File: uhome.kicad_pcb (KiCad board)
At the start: 2 copper layers, 26 x 25.5 mm, 290 parts, among them J1 C2, J2 ANT, U1 Si7006, U2 LPS22HB, U3 EFM8SB10, U4 Si4012, U5 AH1806

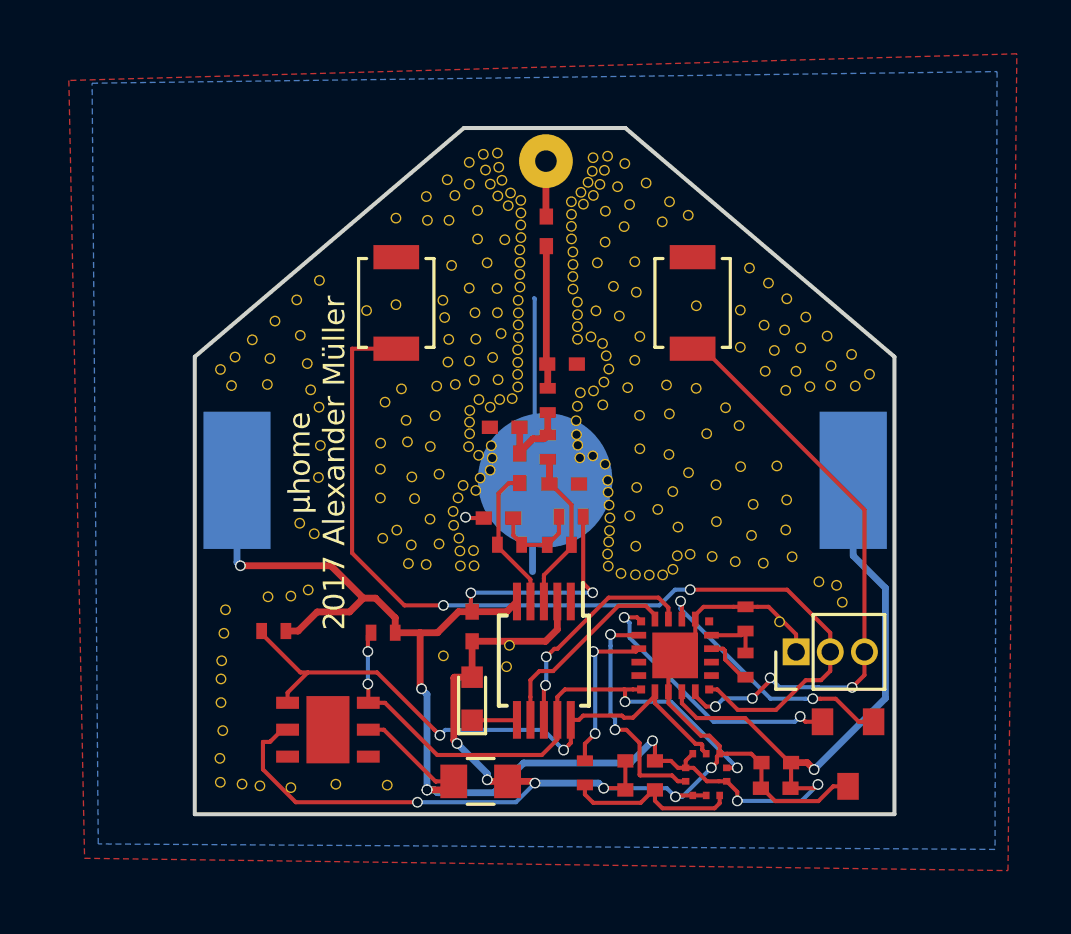
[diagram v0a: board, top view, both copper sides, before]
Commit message: Revision 2
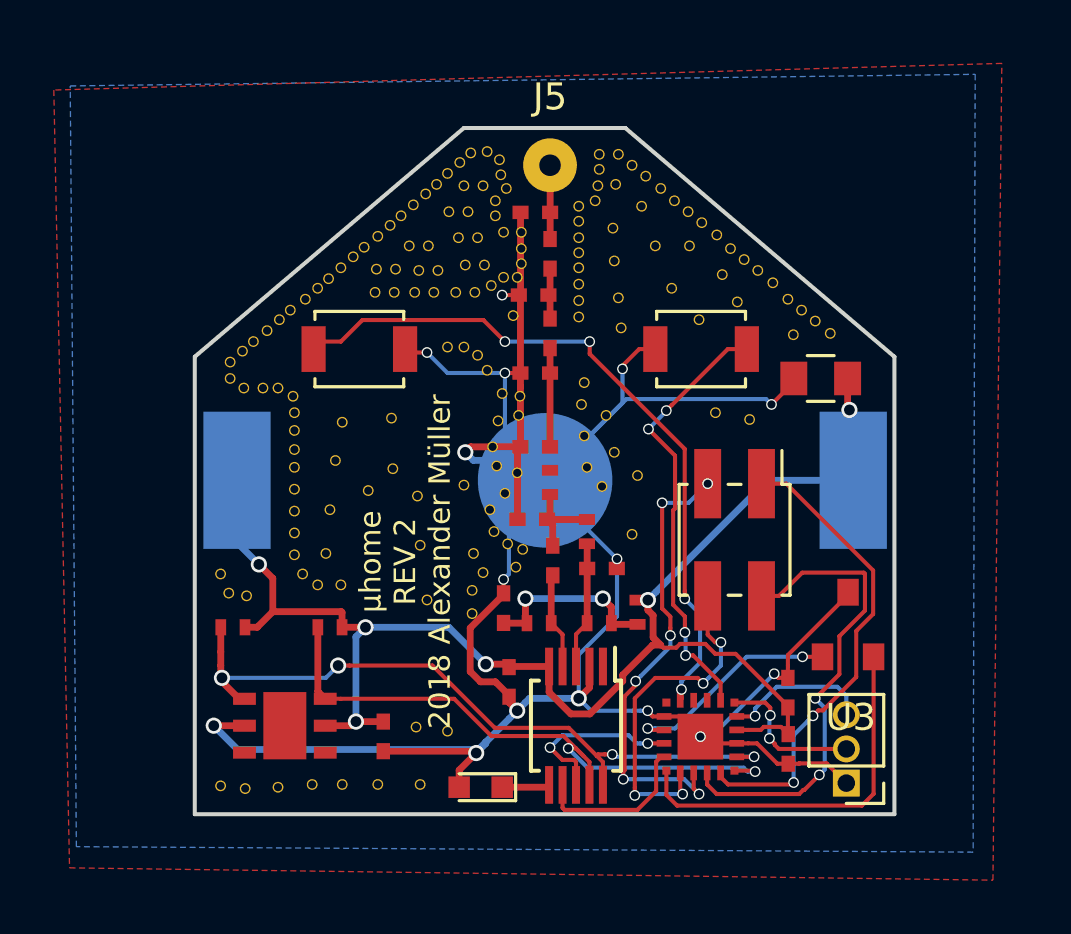
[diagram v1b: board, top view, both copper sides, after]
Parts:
- removed the ? at (173.7, 142.8)
- removed the ? at (152.9, 148.8)
- removed the ? at (159.5, 127.8)
- removed the ? at (169.6, 136.6)
- removed the ? at (169.6, 135.1)
- removed the ? at (168.5, 135.2)
- removed the ? at (168.5, 136.4)
- removed the ? at (168.4, 137.9)
- removed the ? at (168.2, 138.9)
- removed the ? at (169.2, 138.7)
- removed the ? at (169.8, 138.0)
- removed the ? at (170.3, 137.3)
- removed the ? at (152.9, 147.9)
- removed the ? at (171.0, 135.9)
- removed the ? at (171.4, 137.8)
- removed the ? at (172.3, 137.1)
- removed the ? at (171.4, 139.1)
- removed the ? at (172.8, 138.5)
- removed the ? at (172.7, 139.6)
- removed the ? at (170.0, 139.3)
- removed the ? at (168.4, 140.0)
- removed the ? at (169.9, 140.4)
- removed the ? at (170.4, 140.3)
- removed the ? at (153.0, 146.9)
- removed the ? at (171.2, 140.4)
- removed the ? at (172.1, 140.6)
- removed the ? at (173.1, 140.7)
- removed the ? at (175.2, 141.4)
- removed the ? at (176.1, 142.1)
- removed the ? at (175.8, 141.5)
- removed the ? at (174.2, 140.4)
- removed the ? at (174.0, 139.4)
- removed the ? at (174.0, 138.3)
- removed the ? at (173.6, 137.1)
- removed the ? at (153.0, 145.9)
- removed the ? at (172.2, 135.6)
- removed the ? at (171.7, 134.9)
- removed the ? at (170.6, 134.2)
- removed the ? at (169.5, 134.1)
- removed the ? at (168.1, 134.1)
- removed the ? at (167.2, 134.8)
- removed the ? at (161.1, 140.0)
- removed the ? at (160.7, 139.0)
- removed the ? at (160.2, 138.3)
- removed the ? at (160.1, 137.5)
- removed the ? at (153.0, 145.0)
- removed the ? at (161.1, 137.4)
- removed the ? at (160.8, 136.3)
- removed the ? at (159.9, 136.2)
- removed the ? at (159.9, 135.4)
- removed the ? at (160.9, 135.2)
- removed the ? at (161.0, 134.1)
- removed the ? at (159.7, 134.2)
- removed the ? at (159.1, 134.7)
- removed the ? at (158.9, 136.2)
- removed the ? at (158.9, 137.2)
- removed the ? at (153.0, 144.3)
- removed the ? at (158.9, 138.2)
- removed the ? at (159.9, 140.7)
- removed the ? at (159.0, 139.7)
- removed the ? at (159.5, 139.4)
- removed the ? at (160.0, 140.0)
- removed the ? at (160.6, 140.7)
- removed the ? at (156.3, 134.2)
- removed the ? at (156.6, 134.9)
- removed the ? at (156.7, 136.3)
- removed the ? at (156.6, 137.5)
- removed the ? at (153.1, 143.3)
- removed the ? at (155.9, 139.2)
- removed the ? at (156.4, 139.6)
- removed the ? at (162.6, 134.6)
- removed the ? at (162.2, 135.0)
- removed the ? at (162.2, 135.4)
- removed the ? at (162.2, 135.9)
- removed the ? at (162.2, 136.3)
- removed the ? at (162.5, 136.7)
- removed the ? at (167.3, 125.5)
- removed the ? at (167.2, 126.1)
- removed the ? at (153.1, 142.4)
- removed the ? at (167.1, 126.6)
- removed the ? at (166.8, 127.0)
- removed the ? at (162.7, 125.5)
- removed the ? at (162.8, 126.1)
- removed the ? at (163.0, 126.6)
- removed the ? at (163.3, 127.0)
- removed the ? at (163.6, 127.4)
- removed the ? at (166.4, 127.3)
- removed the ? at (163.2, 125.4)
- removed the ? at (163.3, 126.0)
- removed the ? at (156.2, 141.7)
- removed the ? at (163.4, 126.4)
- removed the ? at (163.7, 126.9)
- removed the ? at (166.8, 125.6)
- removed the ? at (166.8, 126.1)
- removed the ? at (166.6, 126.5)
- removed the ? at (166.3, 126.9)
- removed the ? at (169.8, 140.9)
- removed the ? at (169.4, 141.1)
- removed the ? at (168.9, 141.1)
- removed the ? at (168.4, 141.1)
- removed the ? at (155.6, 141.9)
- removed the ? at (167.8, 141.1)
- removed the ? at (167.4, 140.8)
- removed the ? at (167.3, 140.3)
- removed the ? at (167.4, 139.9)
- removed the ? at (167.4, 139.5)
- removed the ? at (167.4, 139.0)
- removed the ? at (167.4, 138.5)
- removed the ? at (167.4, 138.0)
- removed the ? at (167.3, 137.6)
- removed the ? at (167.2, 137.0)
- removed the ? at (161.2, 144.1)
- removed the ? at (154.7, 141.9)
- removed the ? at (166.8, 136.7)
- removed the ? at (166.3, 136.8)
- removed the ? at (166.2, 136.3)
- removed the ? at (166.2, 135.9)
- removed the ? at (166.2, 135.4)
- removed the ? at (166.2, 134.8)
- removed the ? at (166.3, 134.3)
- removed the ? at (166.8, 134.3)
- removed the ? at (167.2, 133.9)
- removed the ? at (167.4, 133.5)
- removed the ? at (170.6, 131.1)
- removed the ? at (167.3, 133.0)
- removed the ? at (167.2, 132.5)
- removed the ? at (166.7, 132.3)
- removed the ? at (166.2, 132.3)
- removed the ? at (166.2, 131.9)
- removed the ? at (166.2, 131.4)
- removed the ? at (166.2, 131.0)
- removed the ? at (166.1, 130.5)
- removed the ? at (166.0, 130.0)
- removed the ? at (166.1, 129.6)
- removed the ? at (159.5, 131.1)
- removed the ? at (166.0, 129.1)
- removed the ? at (166.0, 128.6)
- removed the ? at (166.0, 128.2)
- removed the ? at (166.0, 127.7)
- removed the ? at (166.0, 127.2)
- removed the ? at (164.1, 128.6)
- removed the ? at (164.1, 128.1)
- removed the ? at (164.1, 127.7)
- removed the ? at (164.1, 127.2)
- removed the ? at (164.1, 130.4)
- removed the ? at (158.4, 131.3)
- removed the ? at (164.1, 129.9)
- removed the ? at (164.1, 129.5)
- removed the ? at (164.1, 129.0)
- removed the ? at (164.0, 132.3)
- removed the ? at (164.0, 131.8)
- removed the ? at (164.0, 131.4)
- removed the ? at (164.0, 130.9)
- removed the ? at (164.0, 133.2)
- removed the ? at (164.0, 132.7)
- removed the ? at (164.0, 133.7)
- removed the ? at (155.9, 132.2)
- removed the ? at (164.0, 134.1)
- removed the ? at (163.8, 134.6)
- removed the ? at (163.3, 134.6)
- removed the ? at (163.0, 134.9)
- removed the ? at (162.0, 137.8)
- removed the ? at (162.4, 138.0)
- removed the ? at (163.0, 136.3)
- removed the ? at (163.1, 136.8)
- removed the ? at (163.0, 137.2)
- removed the ? at (162.6, 137.5)
- removed the ? at (156.2, 133.3)
- removed the ? at (161.8, 138.2)
- removed the ? at (161.6, 138.7)
- removed the ? at (161.6, 139.3)
- removed the ? at (161.8, 139.7)
- removed the ? at (162.4, 140.2)
- removed the ? at (161.9, 140.2)
- removed the ? at (161.9, 140.8)
- removed the ? at (162.4, 140.8)
- removed the ? at (154.8, 133.1)
- removed the ? at (154.7, 134.0)
- removed the ? at (153.4, 134.1)
- removed the ? at (153.0, 133.5)
- removed the ? at (163.6, 144.5)
- removed the ? at (153.5, 133.0)
- removed the ? at (154.1, 132.4)
- removed the ? at (155.0, 131.7)
- removed the ? at (155.8, 130.9)
- removed the ? at (156.6, 130.2)
- removed the ? at (174.3, 133.5)
- removed the ? at (173.9, 132.0)
- removed the ? at (173.5, 132.8)
- removed the ? at (175.6, 133.3)
- removed the ? at (174.5, 132.7)
- removed the ? at (163.7, 143.7)
- removed the ? at (173.2, 131.8)
- removed the ? at (172.3, 131.3)
- removed the ? at (172.3, 132.6)
- removed the ? at (173.2, 133.5)
- removed the ? at (174.0, 134.2)
- removed the ? at (174.9, 134.1)
- removed the ? at (175.6, 134.1)
- removed the ? at (176.5, 134.1)
- removed the ? at (177.1, 133.6)
- removed the ? at (176.4, 132.9)
- removed the ? at (159.2, 148.9)
- removed the ? at (175.5, 132.2)
- removed the ? at (174.7, 131.5)
- removed the ? at (174.0, 130.8)
- removed the ? at (173.3, 130.3)
- removed the ? at (172.6, 129.7)
- removed the ? at (168.4, 133.1)
- removed the ? at (168.5, 132.2)
- removed the ? at (167.8, 131.5)
- removed the ? at (166.9, 131.3)
- removed the ? at (167.6, 130.4)
- removed the ? at (157.2, 148.9)
- removed the ? at (168.4, 130.6)
- removed the ? at (167.0, 129.5)
- removed the ? at (167.2, 128.7)
- removed the ? at (168.4, 129.5)
- removed the ? at (168.0, 128.2)
- removed the ? at (167.3, 127.6)
- removed the ? at (167.7, 126.7)
- removed the ? at (168.2, 127.3)
- removed the ? at (169.4, 128.0)
- removed the ? at (170.3, 127.7)
- removed the ? at (155.6, 149.0)
- removed the ? at (169.6, 127.2)
- removed the ? at (168.8, 126.5)
- removed the ? at (168.0, 125.8)
- removed the ? at (161.7, 134.0)
- removed the ? at (161.4, 133.2)
- removed the ? at (161.4, 132.4)
- removed the ? at (162.2, 133.2)
- removed the ? at (162.4, 133.9)
- removed the ? at (163.3, 133.9)
- removed the ? at (163.1, 133.0)
- removed the ? at (154.4, 148.9)
- removed the ? at (162.4, 132.3)
- removed the ? at (163.4, 132.1)
- removed the ? at (163.2, 131.4)
- removed the ? at (162.4, 131.4)
- removed the ? at (161.3, 131.5)
- removed the ? at (161.2, 130.9)
- removed the ? at (162.2, 130.4)
- removed the ? at (163.2, 130.5)
- removed the ? at (162.9, 129.5)
- removed the ? at (161.5, 129.6)
- removed the ? at (153.8, 148.9)
- removed the ? at (162.5, 128.6)
- removed the ? at (163.5, 128.7)
- removed the ? at (162.2, 126.6)
- removed the ? at (161.7, 127.0)
- removed the ? at (160.6, 127.0)
- removed the ? at (161.4, 126.4)
- removed the ? at (162.2, 125.8)
- removed the ? at (162.5, 127.6)
- removed the ? at (161.4, 127.9)
- removed the ? at (160.6, 127.9)
- removed R3: 600, Resistors_SMD:R_0402_NoSilk
- removed R5: 11k, Resistors_SMD:R_0402_NoSilk
- removed REF** (x2): SW_SPST_B3U-1000P, Buttons_Switches_SMD:SW_SPST_B3U-1000P
- removed U5: AH1806, sc59:SC59
- removed eR4: 13k, Resistors_SMD:R_0402_NoSilk
- added ?: , ufqfn:Via, F.Cu at (153.9, 141.9)
- added ?: , ufqfn:Via, F.Cu at (158.8, 148.9)
- added ?: , ufqfn:Via, F.Cu at (160.3, 138.2)
- added ?: , ufqfn:Via, F.Cu at (158.4, 138.0)
- added ?: , ufqfn:Via, F.Cu at (159.4, 137.2)
- added ?: , ufqfn:Via, F.Cu at (159.3, 135.3)
- added ?: , ufqfn:Via, F.Cu at (157.5, 135.4)
- added ?: , ufqfn:Via, F.Cu at (157.2, 136.9)
- added ?: , ufqfn:Via, F.Cu at (157.0, 138.7)
- added ?: , ufqfn:Via, F.Cu at (156.9, 140.3)
- added ?: , ufqfn:Via, F.Cu at (157.4, 141.5)
- added ?: , ufqfn:Via, F.Cu at (156.6, 141.5)
- added ?: , ufqfn:Via, F.Cu at (161.4, 146.9)
- added ?: , ufqfn:Via, F.Cu at (156.0, 141.1)
- added ?: , ufqfn:Via, F.Cu at (155.7, 140.4)
- added ?: , ufqfn:Via, F.Cu at (155.7, 139.5)
- added ?: , ufqfn:Via, F.Cu at (155.7, 138.7)
- added ?: , ufqfn:Via, F.Cu at (155.7, 137.9)
- added ?: , ufqfn:Via, F.Cu at (155.7, 137.1)
- added ?: , ufqfn:Via, F.Cu at (155.7, 136.4)
- added ?: , ufqfn:Via, F.Cu at (155.7, 135.7)
- added ?: , ufqfn:Via, F.Cu at (155.7, 135.1)
- added ?: , ufqfn:Via, F.Cu at (155.7, 134.5)
- added ?: , ufqfn:Via, F.Cu at (160.2, 146.8)
- added ?: , ufqfn:Via, F.Cu at (155.1, 134.2)
- added ?: , ufqfn:Via, F.Cu at (154.5, 134.2)
- added ?: , ufqfn:Via, F.Cu at (153.8, 134.2)
- added ?: , ufqfn:Via, F.Cu at (153.3, 133.8)
- added ?: , ufqfn:Via, F.Cu at (154.2, 132.4)
- added ?: , ufqfn:Via, F.Cu at (153.8, 132.8)
- added ?: , ufqfn:Via, F.Cu at (153.3, 133.2)
- added ?: , ufqfn:Via, F.Cu at (155.5, 131.3)
- added ?: , ufqfn:Via, F.Cu at (155.1, 131.6)
- added ?: , ufqfn:Via, F.Cu at (154.7, 132.0)
- added ?: , ufqfn:Via, F.Cu at (167.6, 136.6)
- added ?: , ufqfn:Via, F.Cu at (157.0, 130.1)
- added ?: , ufqfn:Via, F.Cu at (156.6, 130.5)
- added ?: , ufqfn:Via, F.Cu at (156.1, 130.9)
- added ?: , ufqfn:Via, F.Cu at (158.3, 128.9)
- added ?: , ufqfn:Via, F.Cu at (157.9, 129.3)
- added ?: , ufqfn:Via, F.Cu at (157.4, 129.7)
- added ?: , ufqfn:Via, F.Cu at (159.7, 127.8)
- added ?: , ufqfn:Via, F.Cu at (159.3, 128.1)
- added ?: , ufqfn:Via, F.Cu at (158.8, 128.5)
- added ?: , ufqfn:Via, F.Cu at (161.0, 126.6)
- added ?: , ufqfn:Via, F.Cu at (167.1, 137.8)
- added ?: , ufqfn:Via, F.Cu at (160.6, 126.9)
- added ?: , ufqfn:Via, F.Cu at (160.1, 127.4)
- added ?: , ufqfn:Via, F.Cu at (161.4, 126.2)
- added ?: , ufqfn:Via, F.Cu at (161.8, 125.8)
- added ?: , ufqfn:Via, F.Cu at (162.3, 125.4)
- added ?: , ufqfn:Via, F.Cu at (162.9, 125.4)
- added ?: , ufqfn:Via, F.Cu at (163.3, 125.7)
- added ?: , ufqfn:Via, F.Cu at (163.4, 126.2)
- added ?: , ufqfn:Via, F.Cu at (163.6, 126.7)
- added ?: , ufqfn:Via, F.Cu at (163.2, 127.2)
- added ?: , ufqfn:Via, F.Cu at (166.6, 137.1)
- added ?: , ufqfn:Via, F.Cu at (163.2, 127.8)
- added ?: , ufqfn:Via, F.Cu at (163.5, 128.4)
- added ?: , ufqfn:Via, F.Cu at (166.3, 127.4)
- added ?: , ufqfn:Via, F.Cu at (166.3, 128.0)
- added ?: , ufqfn:Via, F.Cu at (166.3, 128.6)
- added ?: , ufqfn:Via, F.Cu at (166.3, 129.1)
- added ?: , ufqfn:Via, F.Cu at (166.3, 129.7)
- added ?: , ufqfn:Via, F.Cu at (166.3, 130.3)
- added ?: , ufqfn:Via, F.Cu at (166.3, 130.9)
- added ?: , ufqfn:Via, F.Cu at (166.3, 131.5)
- added ?: , ufqfn:Via, F.Cu at (166.5, 135.9)
- added ?: , ufqfn:Via, F.Cu at (163.8, 131.5)
- added ?: , ufqfn:Via, F.Cu at (163.0, 130.4)
- added ?: , ufqfn:Via, F.Cu at (163.5, 130.0)
- added ?: , ufqfn:Via, F.Cu at (164.0, 130.0)
- added ?: , ufqfn:Via, F.Cu at (164.1, 129.5)
- added ?: , ufqfn:Via, F.Cu at (164.1, 129.0)
- added ?: , ufqfn:Via, F.Cu at (164.1, 128.4)
- added ?: , ufqfn:Via, F.Cu at (162.0, 137.8)
- added ?: , ufqfn:Via, F.Cu at (166.4, 134.8)
- added ?: , ufqfn:Via, F.Cu at (166.5, 134.0)
- added ?: , ufqfn:Via, F.Cu at (167.3, 135.2)
- added ?: , ufqfn:Via, F.Cu at (153.3, 141.8)
- added ?: , ufqfn:Via, F.Cu at (168.5, 137.4)
- added ?: , ufqfn:Via, F.Cu at (168.2, 139.6)
- added ?: , ufqfn:Via, F.Cu at (172.6, 135.3)
- added ?: , ufqfn:Via, F.Cu at (171.3, 135.1)
- added ?: , ufqfn:Via, F.Cu at (174.2, 132.2)
- added ?: , ufqfn:Via, F.Cu at (172.2, 131.0)
- added ?: , ufqfn:Via, F.Cu at (170.7, 131.6)
- added ?: , ufqfn:Via, F.Cu at (167.8, 131.9)
- added ?: , ufqfn:Via, F.Cu at (167.7, 130.8)
- added ?: , ufqfn:Via, F.Cu at (169.7, 130.5)
- added ?: , ufqfn:Via, F.Cu at (153.0, 141.1)
- added ?: , ufqfn:Via, F.Cu at (171.6, 129.9)
- added ?: , ufqfn:Via, F.Cu at (170.4, 128.9)
- added ?: , ufqfn:Via, F.Cu at (169.1, 128.9)
- added ?: , ufqfn:Via, F.Cu at (167.6, 129.4)
- added ?: , ufqfn:Via, F.Cu at (167.5, 128.2)
- added ?: , ufqfn:Via, F.Cu at (168.6, 127.4)
- added ?: , ufqfn:Via, F.Cu at (167.6, 126.6)
- added ?: , ufqfn:Via, F.Cu at (174.0, 130.9)
- added ?: , ufqfn:Via, F.Cu at (175.1, 131.7)
- added ?: , ufqfn:Via, F.Cu at (174.5, 131.3)
- added ?: , ufqfn:Via, F.Cu at (153.0, 148.9)
- added ?: , ufqfn:Via, F.Cu at (175.6, 132.1)
- added ?: , ufqfn:Via, F.Cu at (171.9, 129.0)
- added ?: , ufqfn:Via, F.Cu at (172.9, 129.8)
- added ?: , ufqfn:Via, F.Cu at (172.4, 129.4)
- added ?: , ufqfn:Via, F.Cu at (173.5, 130.3)
- added ?: , ufqfn:Via, F.Cu at (169.8, 127.2)
- added ?: , ufqfn:Via, F.Cu at (170.8, 128.0)
- added ?: , ufqfn:Via, F.Cu at (170.3, 127.6)
- added ?: , ufqfn:Via, F.Cu at (171.4, 128.5)
- added ?: , ufqfn:Via, F.Cu at (169.3, 126.7)
- added ?: , ufqfn:Via, F.Cu at (153.9, 149.0)
- added ?: , ufqfn:Via, F.Cu at (168.8, 126.3)
- added ?: , ufqfn:Via, F.Cu at (168.2, 125.9)
- added ?: , ufqfn:Via, F.Cu at (166.9, 127.2)
- added ?: , ufqfn:Via, F.Cu at (167.0, 126.6)
- added ?: , ufqfn:Via, F.Cu at (167.0, 126.0)
- added ?: , ufqfn:Via, F.Cu at (167.7, 125.5)
- added ?: , ufqfn:Via, F.Cu at (167.0, 125.5)
- added ?: , ufqfn:Via, F.Cu at (162.7, 126.6)
- added ?: , ufqfn:Via, F.Cu at (162.0, 126.6)
- added ?: , ufqfn:Via, F.Cu at (162.2, 127.6)
- added ?: , ufqfn:Via, F.Cu at (155.1, 149.0)
- added ?: , ufqfn:Via, F.Cu at (161.4, 127.6)
- added ?: , ufqfn:Via, F.Cu at (160.7, 128.9)
- added ?: , ufqfn:Via, F.Cu at (160.0, 128.9)
- added ?: , ufqfn:Via, F.Cu at (162.5, 128.6)
- added ?: , ufqfn:Via, F.Cu at (161.8, 128.6)
- added ?: , ufqfn:Via, F.Cu at (162.8, 129.6)
- added ?: , ufqfn:Via, F.Cu at (162.1, 129.6)
- added ?: , ufqfn:Via, F.Cu at (161.0, 129.8)
- added ?: , ufqfn:Via, F.Cu at (160.3, 129.8)
- added ?: , ufqfn:Via, F.Cu at (159.5, 129.7)
- added ?: , ufqfn:Via, F.Cu at (156.4, 148.9)
- added ?: , ufqfn:Via, F.Cu at (158.8, 129.7)
- added ?: , ufqfn:Via, F.Cu at (159.4, 130.6)
- added ?: , ufqfn:Via, F.Cu at (158.7, 130.6)
- added ?: , ufqfn:Via, F.Cu at (160.9, 130.6)
- added ?: , ufqfn:Via, F.Cu at (160.2, 130.6)
- added ?: , ufqfn:Via, F.Cu at (161.7, 130.6)
- added ?: , ufqfn:Via, F.Cu at (162.4, 130.6)
- added ?: , ufqfn:Via, F.Cu at (161.4, 132.6)
- added ?: , ufqfn:Via, F.Cu at (162.0, 132.6)
- added ?: , ufqfn:Via, F.Cu at (162.5, 132.9)
- added ?: , ufqfn:Via, F.Cu at (157.5, 148.9)
- added ?: , ufqfn:Via, F.Cu at (162.9, 133.5)
- added ?: , ufqfn:Via, F.Cu at (163.4, 134.4)
- added ?: , ufqfn:Via, F.Cu at (164.1, 134.5)
- added ?: , ufqfn:Via, F.Cu at (164.0, 135.2)
- added ?: , ufqfn:Via, F.Cu at (163.3, 135.4)
- added ?: , ufqfn:Via, F.Cu at (163.1, 136.3)
- added ?: , ufqfn:Via, F.Cu at (163.2, 137.1)
- added ?: , ufqfn:Via, F.Cu at (164.0, 137.3)
- added ?: , ufqfn:Via, F.Cu at (163.5, 138.1)
- added ?: , ufqfn:Via, F.Cu at (163.0, 138.7)
- added ?: , ufqfn:Via, F.Cu at (160.4, 148.9)
- added ?: , ufqfn:Via, F.Cu at (163.1, 139.5)
- added ?: , ufqfn:Via, F.Cu at (163.6, 140.0)
- added ?: , ufqfn:Via, F.Cu at (164.2, 140.2)
- added ?: , ufqfn:Via, F.Cu at (163.9, 140.8)
- added ?: , ufqfn:Via, F.Cu at (162.7, 141.0)
- added ?: , ufqfn:Via, F.Cu at (162.3, 142.5)
- added ?: , ufqfn:Via, F.Cu at (162.3, 141.7)
- added ?: , ufqfn:Via, F.Cu at (162.4, 140.3)
- added ?: , ufqfn:Via, F.Cu at (160.4, 140.0)
- added ?: , ufqfn:Via, F.Cu at (160.6, 142.0)
- added C13: CM3 (2.7pF), Capacitors_SMD:C_0402_NoSilk, F.Cu at (163.5, 142.3)
- added J3: Conn_01x04, Pin_Headers:Pin_Header_Straight_2x02_Pitch2.00mm_SMD, F.Cu at (172.1, 139.8)
- added J4: Conn_01x02, Buttons_Switches_SMD:SW_SPST_B3U-1000P, F.Cu at (158.1, 132.7)
- added J5: ANT, Wire_Pads:SolderWirePad_single_0-8mmDrill, F.Cu at (165.2, 125.9)
- added L6: LM4 (16 nH), Resistors_SMD:R_0402_NoSilk, F.Cu at (164.8, 142.9)
- added L7: LM1 (220 nH), Resistors_SMD:R_0402_NoSilk, F.Cu at (168.5, 142.5)
- C1, C4: value 0.1µ -> 1µ
- C10: value CM1 -> CM5 (6.8pF)
- C11: value CM2 -> CM1 (4.3pF)
- C12: value CM3 -> CM2 (1.8 pF)
- C3: value 1µ -> 0.1µ
- C5: value 1µ -> 4.5pF
- C6: value CC1 -> 15pF
- C7: value 20µ -> 4.5pF; footprint Capacitors_SMD:C_0805 -> Capacitors_SMD:C_0402_NoSilk
- C8: value CM6 -> 20µ; footprint Capacitors_SMD:C_0402_NoSilk -> Capacitors_SMD:C_0805
- C9: value CM5 -> CM6 (6.8pF)
- J2: value ANT -> Conn_01x02; footprint Wire_Pads:SolderWirePad_single_0-8mmDrill -> Buttons_Switches_SMD:SW_SPST_B3U-1000P
- L1: value LM5 -> 30nH; footprint Resistors_SMD:R_0402_NoSilk -> Capacitors_SMD:C_0402_NoSilk
- L2: value LM3 -> 30nH; footprint Resistors_SMD:R_0402_NoSilk -> Capacitors_SMD:C_0402_NoSilk
- L3: value LM2 -> LM5 (18nH)
- L4: value LM4 -> LM3 (56 nH)
- L5: value LM1 -> LM2 (16 nH)
- U2: value LPS22HB -> EFM8SB10; footprint ufqfn:HLGA-10L -> ufqfn:20-UFQFN
- U3: value EFM8SB10 -> AH1806; footprint ufqfn:20-UFQFN -> sc59:SC59
- moved C5 15.6 mm to (164.7, 127.6), turned to 180 degrees
- moved C7 15.3 mm to (164.7, 133.6)
- moved C3 14.7 mm to (159.0, 147.1), turned to 270 degrees
- moved C4 10.4 mm to (163.7, 145.1), turned to 90 degrees
- moved C8 9.63 mm to (175.3, 133.8)
- moved J2 9.06 mm to (170.8, 132.7), turned to 180 degrees
- moved C2 6.57 mm to (174.0, 145.5), turned to 90 degrees
- moved U3 6.53 mm to (176.3, 143.0), turned to 0 degrees
- moved C1 5.52 mm to (174.1, 147.6), turned to 270 degrees
- moved L1 5.45 mm to (165.2, 129.2)
- moved J1 5.22 mm to (176.2, 148.8), turned to 180 degrees
- moved C11 4.82 mm to (167.1, 140.9), turned to 180 degrees
- moved L2 4.23 mm to (165.2, 132.1)
- moved L5 4.09 mm to (167.0, 142.9), turned to 0 degrees
- moved D1 3.30 mm to (162.6, 149.0), turned to 180 degrees
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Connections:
- C10 pad 1: GND -> Net-(C10-Pad1)
- C10 pad 2: ANT_M -> GND
- C11 pad 1: Net-(C11-Pad1) -> GND
- C11 pad 2: ANT_P -> ANT_M
- C12 pad 1: Net-(C12-Pad1) -> Net-(C10-Pad1)
- C12 pad 2: GND -> ANT_P
- C2 pad 1: GND -> +BATT
- C2 pad 2: LPS_PWR -> GND
- C4 pad 1: +BATT -> GND
- C4 pad 2: GND -> +BATT
- C5 pad 1: GND -> Net-(C5-Pad1)
- C5 pad 2: +BATT -> GND
- C6 pad 2: Net-(C6-Pad2) -> GND
- C7 pad 1: GND -> Net-(C7-Pad1)
- C7 pad 2: +BATT -> GND
- C8 pad 1: Net-(C6-Pad1) -> GND
- C8 pad 2: GND -> +BATT
- C9 pad 1: Net-(C11-Pad1) -> Net-(C7-Pad1)
- J2 pad 1: Net-(C6-Pad2) -> Net-(J2-Pad1)
- L1 pad 1: Net-(C11-Pad1) -> Net-(C6-Pad1)
- L1 pad 2: Net-(C6-Pad1) -> Net-(C5-Pad1)
- L2 pad 1: ANT_M -> Net-(C7-Pad1)
- L2 pad 2: Net-(C11-Pad1) -> Net-(C6-Pad1)
- L3 pad 1: ANT_M -> Net-(C10-Pad1)
- L3 pad 2: Net-(C12-Pad1) -> Net-(C7-Pad1)
- L4 pad 1: Net-(C12-Pad1) -> ANT_M
- L4 pad 2: ANT_P -> Net-(C10-Pad1)
- L5 pad 1: +BATT -> ANT_M
- L5 pad 2: Net-(C12-Pad1) -> Net-(C13-Pad1)
- U2 pad 1: +BATT -> I2C_SCL
- U2 pad 10: LPS_PWR -> Net-(J4-Pad2)
- U2 pad 2: I2C_SCL -> I2C_SDA
- U2 pad 4: I2C_SDA -> +BATT
- U2 pad 5: +BATT -> Net-(J1-Pad3)
- U2 pad 6: +BATT -> Net-(J1-Pad2)
- U2 pad 7: LPS_IRQ -> Net-(J2-Pad1)
- U2 pad 8: GND -> (no net)
- U2 pad 9: GND -> (no net)
- U3 pad 1: I2C_SCL -> Net-(U2-Pad13)
- U3 pad 2: I2C_SDA -> GND
- U3 pad 3: GND -> Net-(U2-Pad16)
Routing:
- net GND: track 65.6 -> 108.3 mm, vias 8 -> 15
- net Net-(J1-Pad2): track 35.6 -> 5.61 mm
- net Net-(J4-Pad2): track 0.00 -> 26.4 mm, vias 0 -> 4
- net +BATT: track 77.1 -> 57.5 mm, vias 10 -> 6
- net Net-(J3-Pad2): track 0.00 -> 17.7 mm, vias 0 -> 2
- net Net-(J3-Pad1): track 0.00 -> 17.7 mm, vias 0 -> 2
- net Net-(J3-Pad3): track 0.00 -> 17.0 mm, vias 0 -> 6
- net Net-(J1-Pad3): track 22.4 -> 5.54 mm, vias 4 -> 1
- net Net-(J2-Pad1): track 0.00 -> 16.3 mm, vias 0 -> 4
- net Net-(U2-Pad16): track 0.00 -> 14.0 mm
- net Net-(J3-Pad4): track 0.00 -> 13.0 mm, vias 0 -> 4
- net Net-(U3-Pad16): track 10.2 -> 0.00 mm, vias 2 -> 0
- net Net-(U3-Pad13): track 9.88 -> 0.00 mm, vias 2 -> 0
- net LPS_IRQ: track 8.79 -> 0.00 mm, vias 2 -> 0
- net Net-(U2-Pad13): track 0.00 -> 8.23 mm, vias 0 -> 2
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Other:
- board text added: "µhome REV 2 2018 Alexander Müller"
- board text removed: "µhome 2017 Alexander Müller"
